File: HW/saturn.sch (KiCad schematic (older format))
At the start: 0 parts

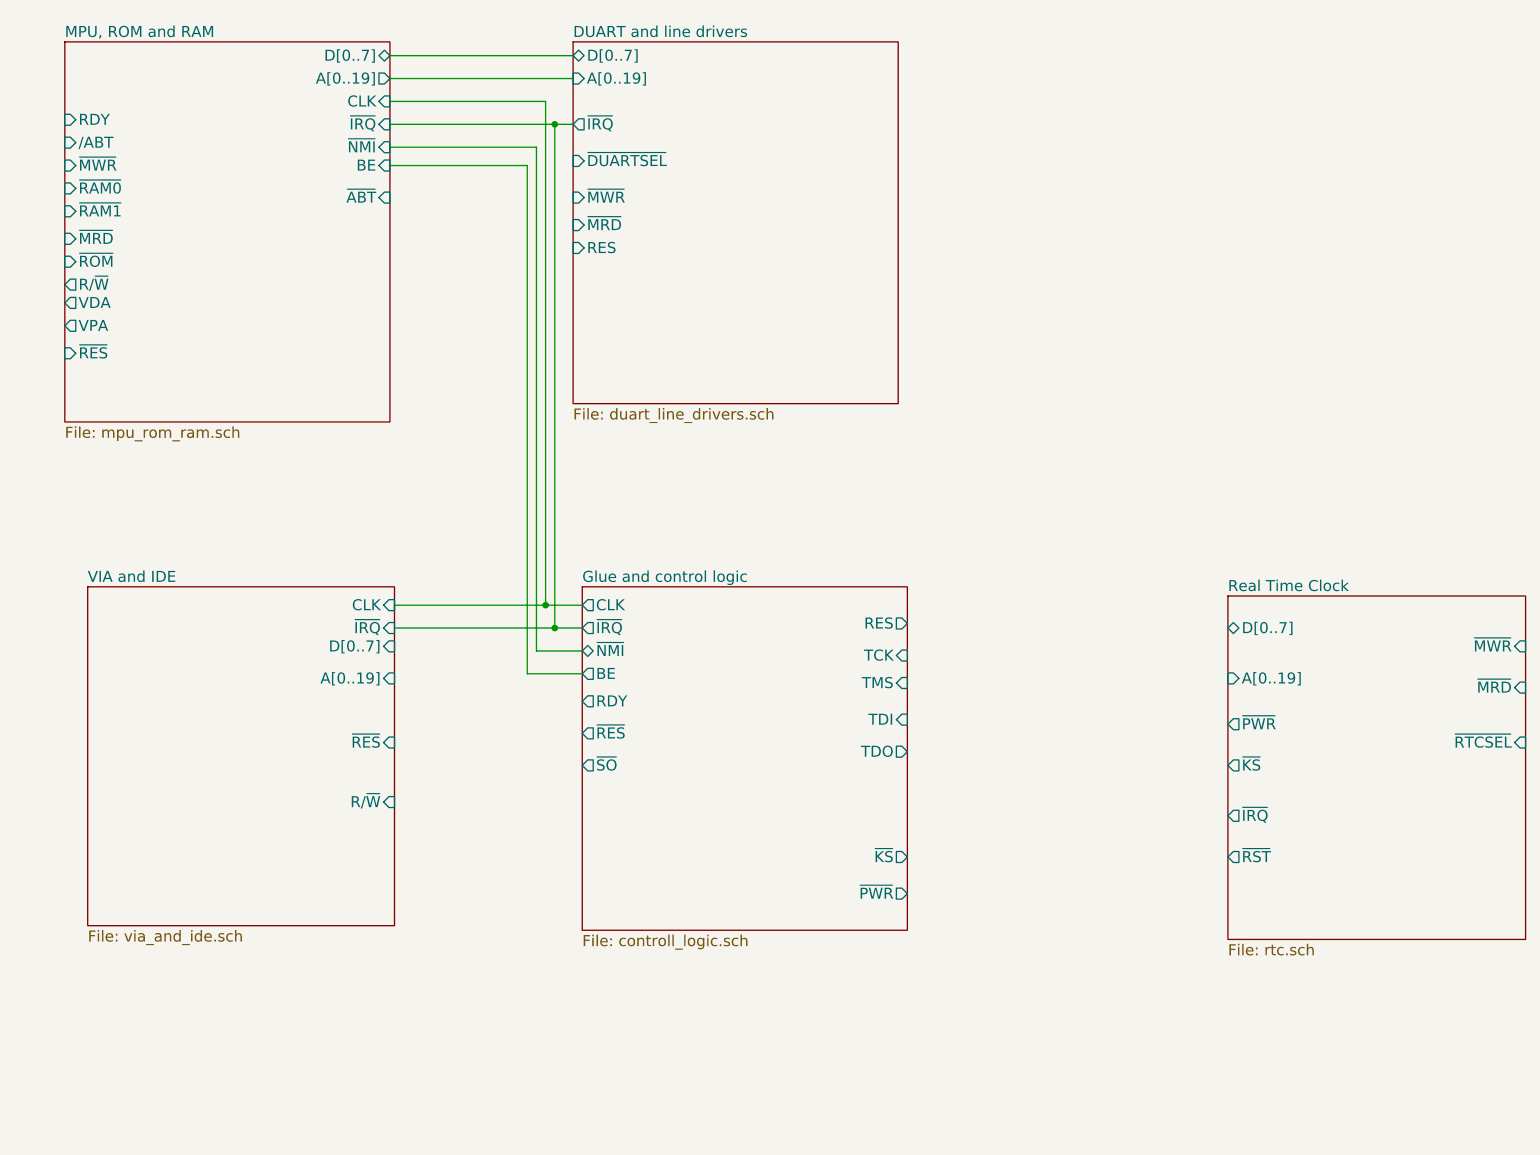
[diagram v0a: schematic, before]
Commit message: ABEL code passes compilation, no tests though. Small changes to schema
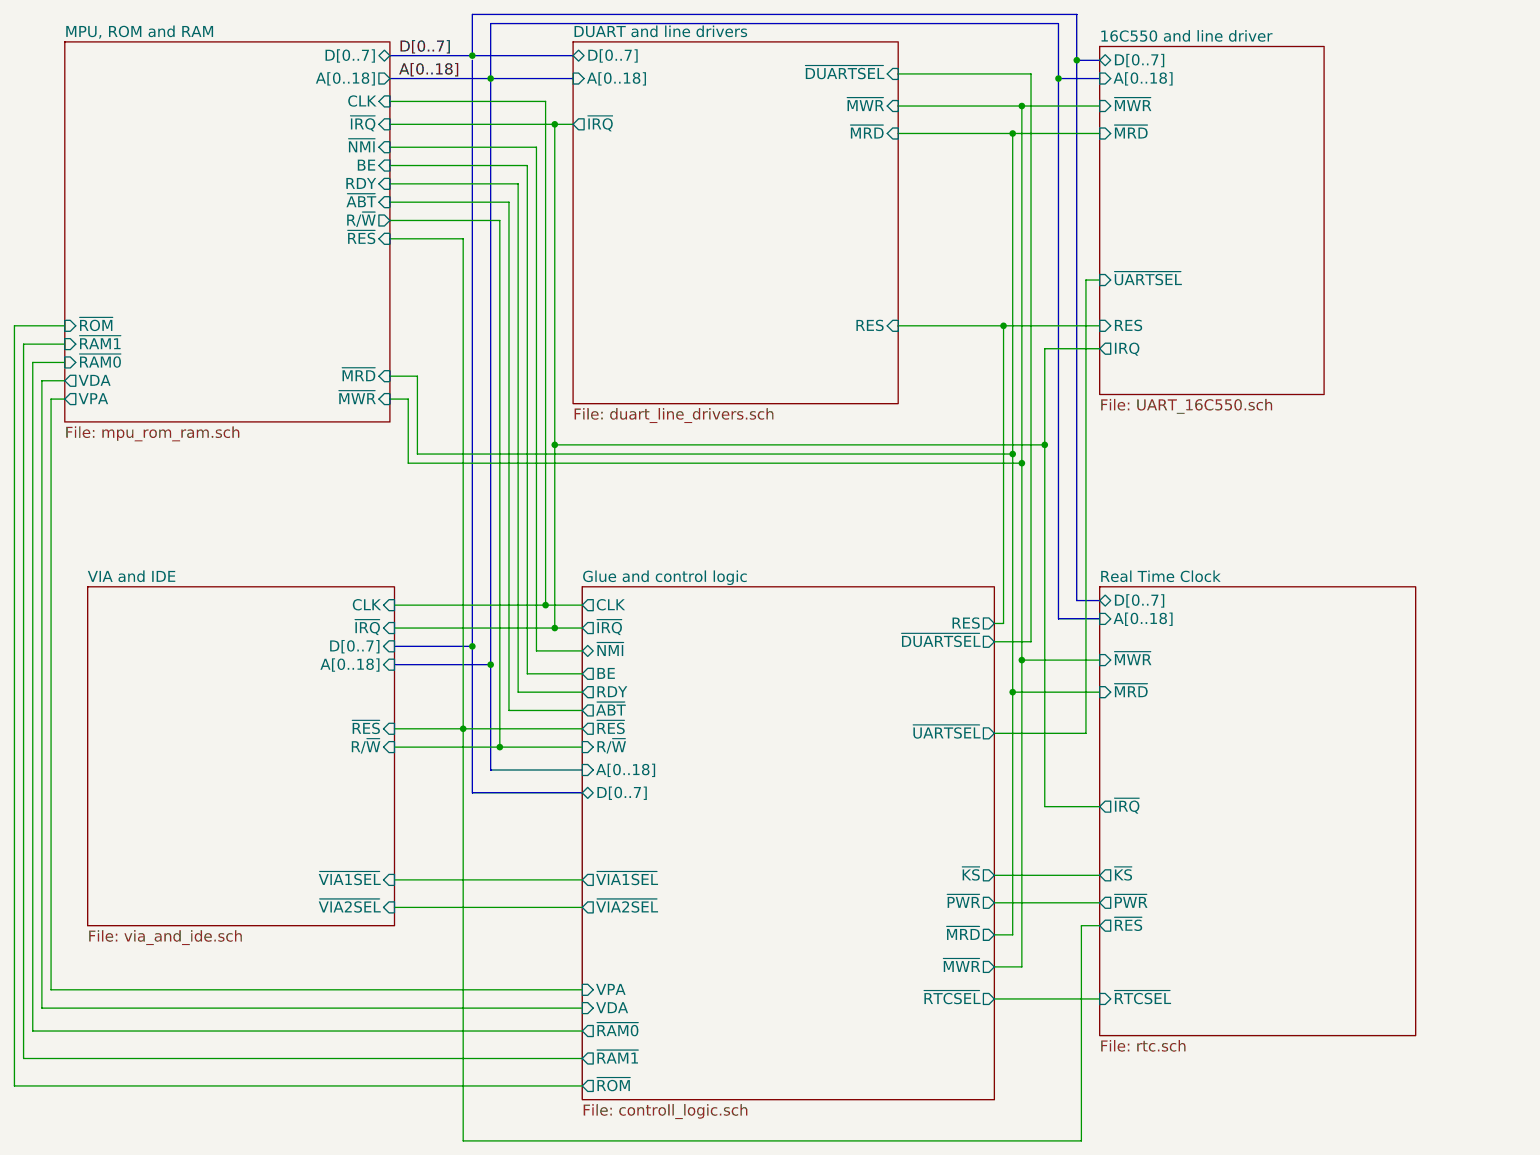
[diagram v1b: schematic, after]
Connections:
- net labels added: A[0..18], D[0..7]
- wire segments 15 -> 74
